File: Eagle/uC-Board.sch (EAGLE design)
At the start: 16 parts, among them IC1 7805T, J1 SWITCHES, J2 ROTARY, J3 DISPLAY, J4 ICOM CIV, J5 PTT IN, J6 YAESU CAT, J7 PTT OUT, J8 PWR IN, Q1 BC557

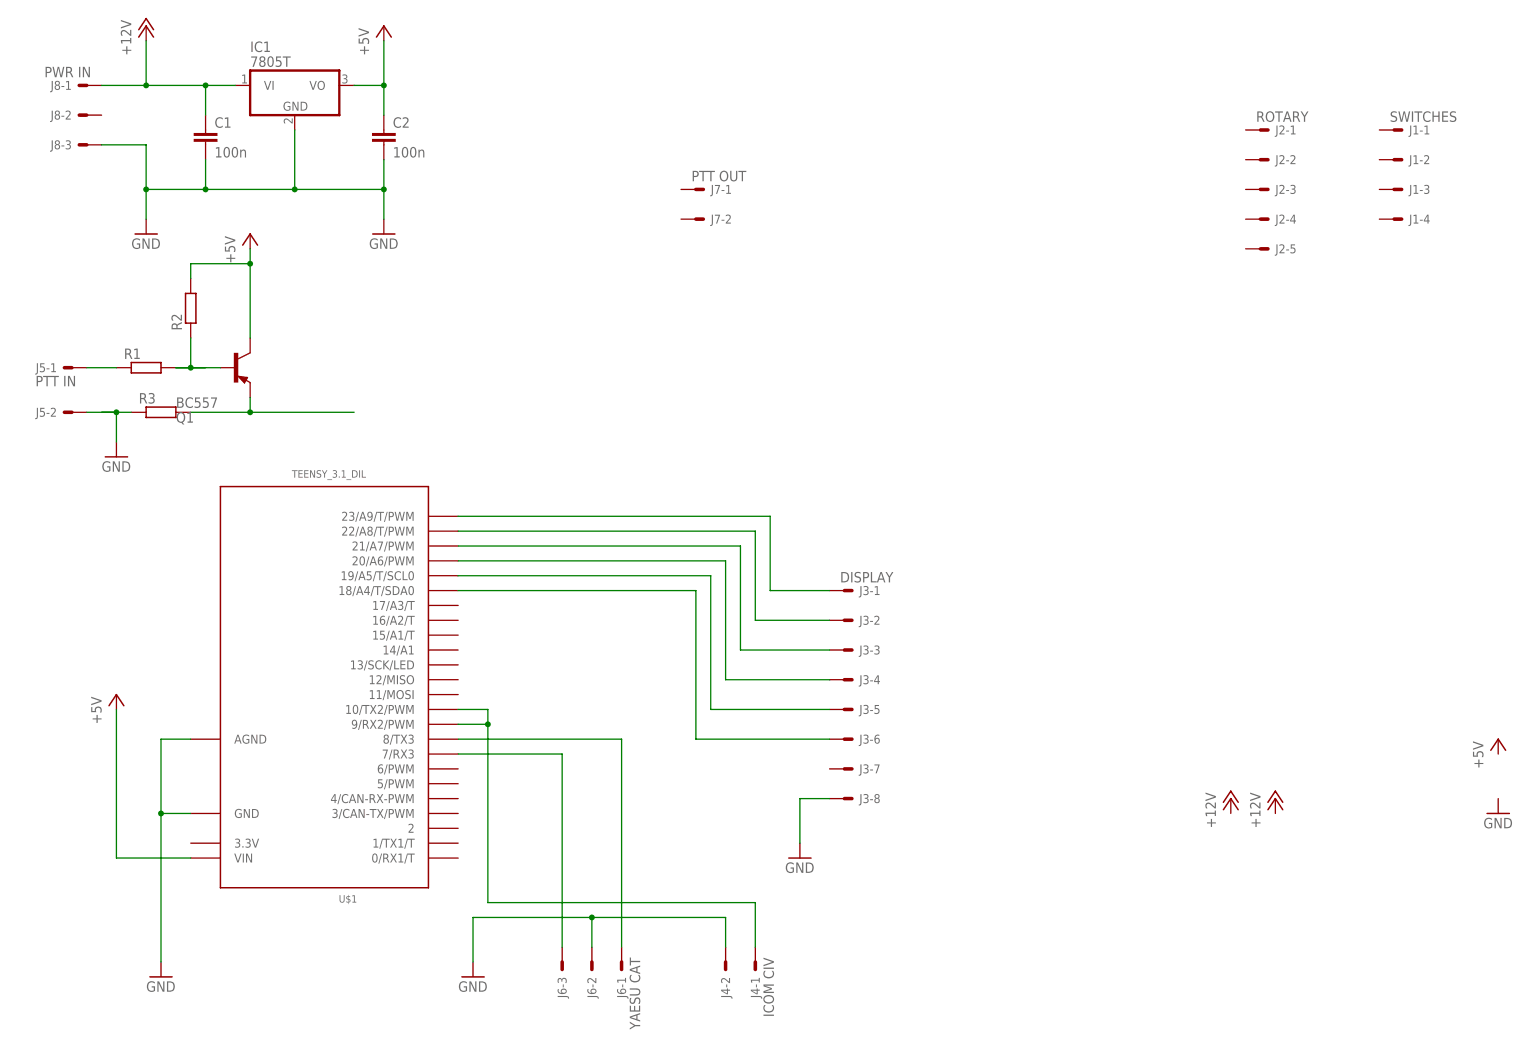
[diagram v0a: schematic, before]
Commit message: added more components, corrections
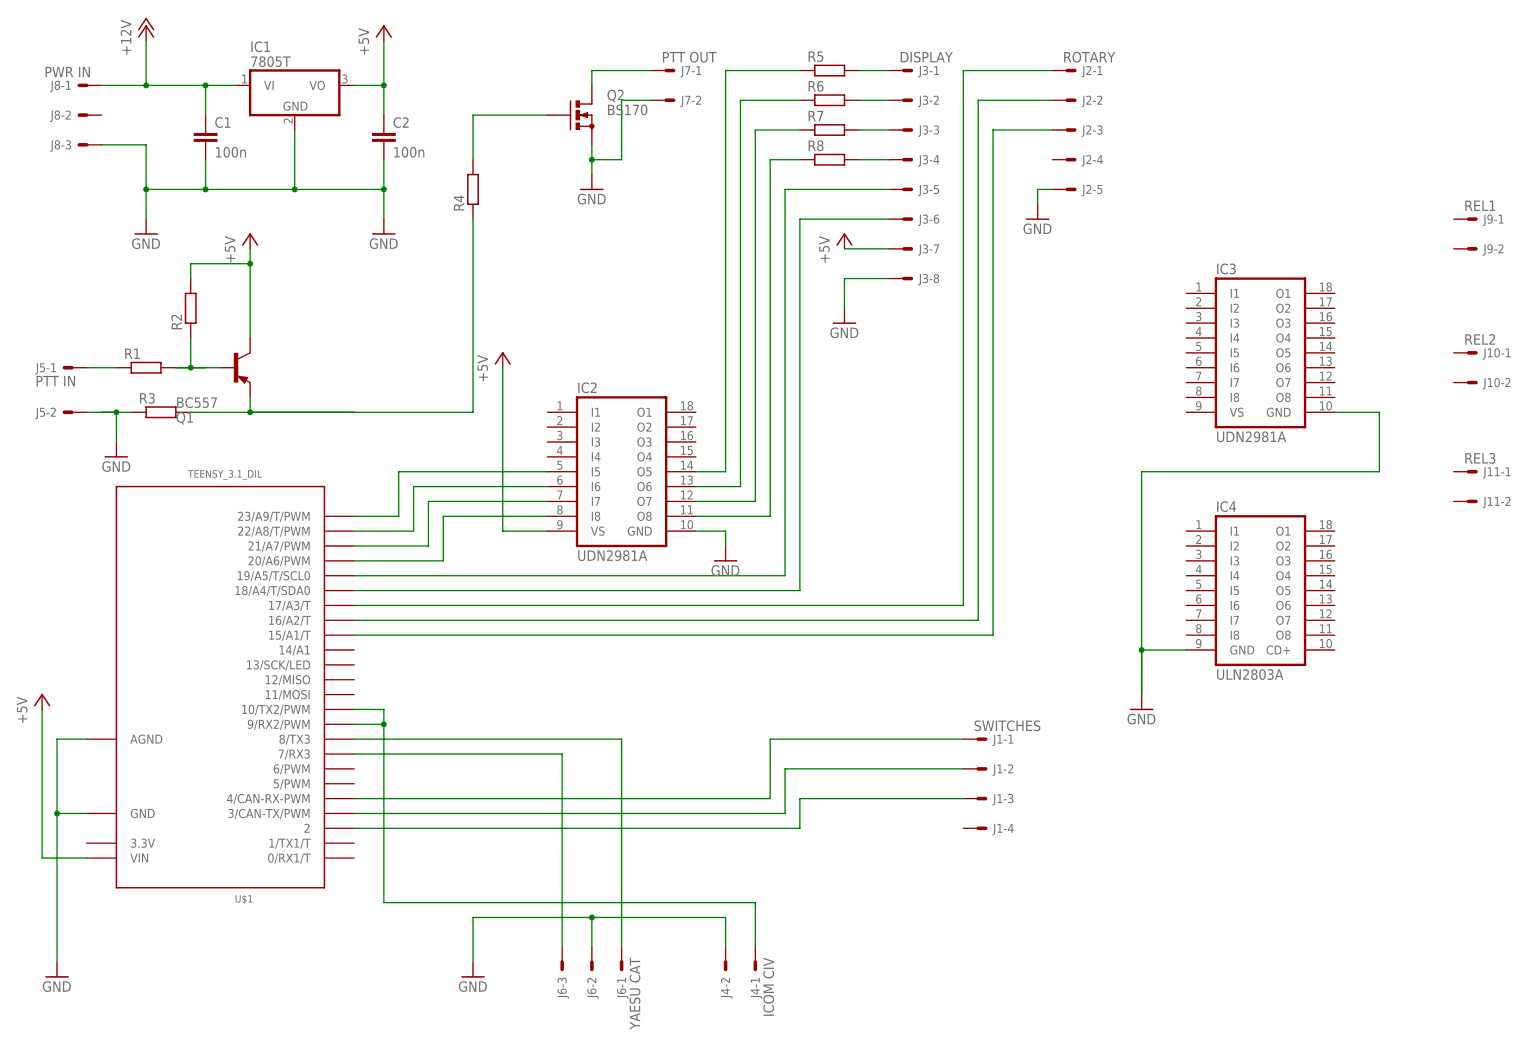
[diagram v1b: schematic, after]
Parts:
- added IC2, IC3: UDN2981A, uln-udn:UDN2981A
- added IC4: ULN2803A, uln-udn:ULN2803A
- added J10: REL2, con-molex:22-27-2021-02
- added J11: REL3, con-molex:22-27-2021-02
- added J9: REL1, con-molex:22-27-2021-02
- added Q2: BS170, transistor-small-signal:BS170
- added R4, R5, R6, R7, R8: (no value), rcl:R-EU_0207/10
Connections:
- new net N$13: J1-1.S, U$1.4/CAN-RX-PWM
- new net N$14: Q2.G, R4.2
- new net N$15: J7-1.S, Q2.D
- new net N$16: J2-1.S, U$1.17/A3/T
- new net N$17: J2-2.S, U$1.16/A2/T
- new net N$18: J2-3.S, U$1.15/A1/T
- new net N$19: J1-2.S, U$1.3/CAN-TX/PWM
- new net N$20: J1-3.S, U$1.2
- new net N$21: IC2.I5, U$1.23/A9/T/PWM
- new net N$22: IC2.I6, U$1.22/A8/T/PWM
- new net N$23: IC2.I7, U$1.21/A7/PWM
- new net N$24: IC2.I8, U$1.20/A6/PWM
- new net N$25: J3-4.S, R8.2
- new net N$26: J3-3.S, R7.2
- new net N$27: J3-2.S, R6.2
- new net N$28: J3-1.S, R5.2
- net +5V: now also IC2.VS, J3-7.S
- net GND: now also IC2.GND, IC3.GND, IC4.GND, J2-5.S, J7-2.S, Q2.S
- net N$11: now also R4.1
- net N$3: now also IC2.O8, R8.1; no longer J3-4.S, U$1.20/A6/PWM
- net N$7: now also IC2.O7, R7.1; no longer J3-3.S, U$1.21/A7/PWM
- net N$8: now also IC2.O6, R6.1; no longer J3-2.S, U$1.22/A8/T/PWM
- net N$9: now also IC2.O5, R5.1; no longer J3-1.S, U$1.23/A9/T/PWM
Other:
- moved on the sheet: J1-1, J1-2, J1-3, J1-4, J2-1, J2-2, J2-3, J2-4, J2-5, J3-1, J3-2, J3-3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
